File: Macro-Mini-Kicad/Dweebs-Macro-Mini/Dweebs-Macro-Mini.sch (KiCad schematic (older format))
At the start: 57 parts, among them U1 ProMicro

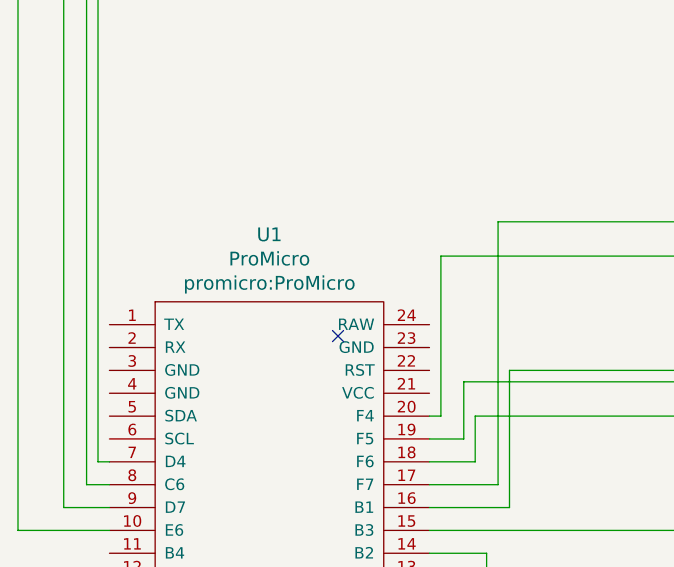
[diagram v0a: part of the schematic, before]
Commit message: more crap
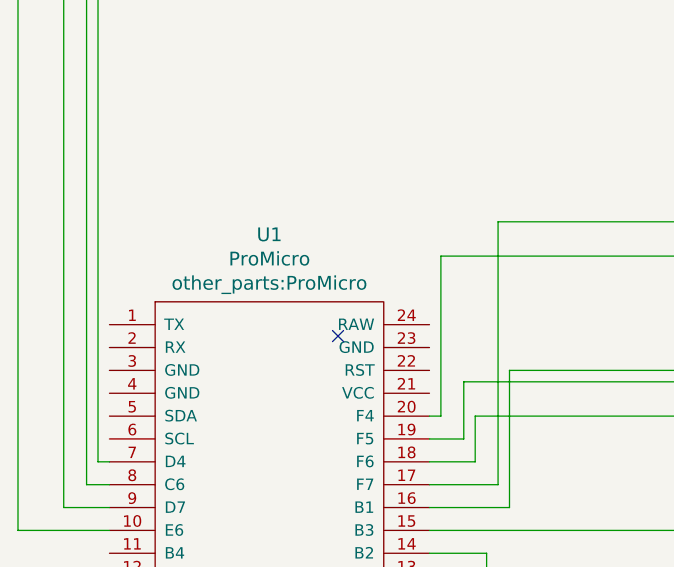
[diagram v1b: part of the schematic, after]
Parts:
- MX1, MX10, MX11, MX12, MX13, MX14, MX15, MX16, MX17, MX18, MX19, MX2, MX20, MX21, MX22, MX23, MX24, MX25, MX26, MX27, MX28, MX3, MX4, MX5, MX6, MX7, MX8, MX9: footprint MX_Alps_Hybrid:MX-1U-NoLED -> kbd:CherryMX_1u
- U1: footprint promicro:ProMicro -> other_parts:ProMicro
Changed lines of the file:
@@
 EESchema Schematic File Version 4
+LIBS:Dweebs-Macro-Mini-cache
 EELAYER 30 0
 EELAYER END
@@
 F 0 "MX1" H 4833 2073 60  0000 C CNN
 F 1 "MX-NoLED" H 4833 1999 20  0000 C CNN
-F 2 "MX_Alps_Hybrid:MX-1U-NoLED" H 4175 1825 60  0001 C CNN
+F 2 "kbd:CherryMX_1u" H 4175 1825 60  0001 C CNN
 F 3 "" H 4175 1825 60  0001 C CNN
 	1    4800 1850
@@
 F 0 "MX2" H 5233 2073 60  0000 C CNN
 F 1 "MX-NoLED" H 5233 1999 20  0000 C CNN
-F 2 "MX_Alps_Hybrid:MX-1U-NoLED" H 4575 1825 60  0001 C CNN
+F 2 "kbd:CherryMX_1u" H 4575 1825 60  0001 C CNN
 F 3 "" H 4575 1825 60  0001 C CNN
 	1    5200 1850
@@
 F 0 "MX3" H 5633 2073 60  0000 C CNN
 F 1 "MX-NoLED" H 5633 1999 20  0000 C CNN
-F 2 "MX_Alps_Hybrid:MX-1U-NoLED" H 4975 1825 60  0001 C CNN
+F 2 "kbd:CherryMX_1u" H 4975 1825 60  0001 C CNN
 F 3 "" H 4975 1825 60  0001 C CNN
 	1    5600 1850
@@
 F 0 "MX4" H 6033 2073 60  0000 C CNN
 F 1 "MX-NoLED" H 6033 1999 20  0000 C CNN
-F 2 "MX_Alps_Hybrid:MX-1U-NoLED" H 5375 1825 60  0001 C CNN
+F 2 "kbd:CherryMX_1u" H 5375 1825 60  0001 C CNN
 F 3 "" H 5375 1825 60  0001 C CNN
 	1    6000 1850
@@
 F 0 "MX5" H 6433 2073 60  0000 C CNN
 F 1 "MX-NoLED" H 6433 1999 20  0000 C CNN
-F 2 "MX_Alps_Hybrid:MX-1U-NoLED" H 5775 1825 60  0001 C CNN
+F 2 "kbd:CherryMX_1u" H 5775 1825 60  0001 C CNN
 F 3 "" H 5775 1825 60  0001 C CNN
 	1    6400 1850
@@
 F 0 "MX6" H 6833 2073 60  0000 C CNN
 F 1 "MX-NoLED" H 6833 1999 20  0000 C CNN
-F 2 "MX_Alps_Hybrid:MX-1U-NoLED" H 6175 1825 60  0001 C CNN
+F 2 "kbd:CherryMX_1u" H 6175 1825 60  0001 C CNN
 F 3 "" H 6175 1825 60  0001 C CNN
 	1    6800 1850
@@
 F 0 "MX7" H 7233 2073 60  0000 C CNN
 F 1 "MX-NoLED" H 7233 1999 20  0000 C CNN
-F 2 "MX_Alps_Hybrid:MX-1U-NoLED" H 6575 1825 60  0001 C CNN
+F 2 "kbd:CherryMX_1u" H 6575 1825 60  0001 C CNN
 F 3 "" H 6575 1825 60  0001 C CNN
 	1    7200 1850
@@
 F 0 "MX8" H 4833 2723 60  0000 C CNN
 F 1 "MX-NoLED" H 4833 2649 20  0000 C CNN
-F 2 "MX_Alps_Hybrid:MX-1U-NoLED" H 4175 2475 60  0001 C CNN
+F 2 "kbd:CherryMX_1u" H 4175 2475 60  0001 C CNN
 F 3 "" H 4175 2475 60  0001 C CNN
 	1    4800 2500
@@
 F 0 "MX9" H 5233 2723 60  0000 C CNN
 F 1 "MX-NoLED" H 5233 2649 20  0000 C CNN
-F 2 "MX_Alps_Hybrid:MX-1U-NoLED" H 4575 2475 60  0001 C CNN
+F 2 "kbd:CherryMX_1u" H 4575 2475 60  0001 C CNN
 F 3 "" H 4575 2475 60  0001 C CNN
 	1    5200 2500
@@
 F 0 "MX10" H 5633 2723 60  0000 C CNN
 F 1 "MX-NoLED" H 5633 2649 20  0000 C CNN
-F 2 "MX_Alps_Hybrid:MX-1U-NoLED" H 4975 2475 60  0001 C CNN
+F 2 "kbd:CherryMX_1u" H 4975 2475 60  0001 C CNN
 F 3 "" H 4975 2475 60  0001 C CNN
 	1    5600 2500
@@
 F 0 "MX11" H 6033 2723 60  0000 C CNN
 F 1 "MX-NoLED" H 6033 2649 20  0000 C CNN
-F 2 "MX_Alps_Hybrid:MX-1U-NoLED" H 5375 2475 60  0001 C CNN
+F 2 "kbd:CherryMX_1u" H 5375 2475 60  0001 C CNN
 F 3 "" H 5375 2475 60  0001 C CNN
 	1    6000 2500
@@
 F 0 "MX12" H 6433 2723 60  0000 C CNN
 F 1 "MX-NoLED" H 6433 2649 20  0000 C CNN
-F 2 "MX_Alps_Hybrid:MX-1U-NoLED" H 5775 2475 60  0001 C CNN
+F 2 "kbd:CherryMX_1u" H 5775 2475 60  0001 C CNN
 F 3 "" H 5775 2475 60  0001 C CNN
 	1    6400 2500
@@
 F 0 "MX13" H 6833 2723 60  0000 C CNN
 F 1 "MX-NoLED" H 6833 2649 20  0000 C CNN
-F 2 "MX_Alps_Hybrid:MX-1U-NoLED" H 6175 2475 60  0001 C CNN
+F 2 "kbd:CherryMX_1u" H 6175 2475 60  0001 C CNN
 F 3 "" H 6175 2475 60  0001 C CNN
 	1    6800 2500
@@
 F 0 "MX14" H 4833 3423 60  0000 C CNN
 F 1 "MX-NoLED" H 4833 3349 20  0000 C CNN
-F 2 "MX_Alps_Hybrid:MX-1U-NoLED" H 4175 3175 60  0001 C CNN
+F 2 "kbd:CherryMX_1u" H 4175 3175 60  0001 C CNN
 F 3 "" H 4175 3175 60  0001 C CNN
 	1    4800 3200
@@
 F 0 "MX15" H 5233 3423 60  0000 C CNN
 F 1 "MX-NoLED" H 5233 3349 20  0000 C CNN
-F 2 "MX_Alps_Hybrid:MX-1U-NoLED" H 4575 3175 60  0001 C CNN
+F 2 "kbd:CherryMX_1u" H 4575 3175 60  0001 C CNN
 F 3 "" H 4575 3175 60  0001 C CNN
 	1    5200 3200
@@
 F 0 "MX16" H 5633 3423 60  0000 C CNN
 F 1 "MX-NoLED" H 5633 3349 20  0000 C CNN
-F 2 "MX_Alps_Hybrid:MX-1U-NoLED" H 4975 3175 60  0001 C CNN
+F 2 "kbd:CherryMX_1u" H 4975 3175 60  0001 C CNN
 F 3 "" H 4975 3175 60  0001 C CNN
 	1    5600 3200
@@
 F 0 "MX17" H 6033 3423 60  0000 C CNN
 F 1 "MX-NoLED" H 6033 3349 20  0000 C CNN
-F 2 "MX_Alps_Hybrid:MX-1U-NoLED" H 5375 3175 60  0001 C CNN
+F 2 "kbd:CherryMX_1u" H 5375 3175 60  0001 C CNN
 F 3 "" H 5375 3175 60  0001 C CNN
 	1    6000 3200
@@
 F 0 "MX18" H 6433 3423 60  0000 C CNN
 F 1 "MX-NoLED" H 6433 3349 20  0000 C CNN
-F 2 "MX_Alps_Hybrid:MX-1U-NoLED" H 5775 3175 60  0001 C CNN
+F 2 "kbd:CherryMX_1u" H 5775 3175 60  0001 C CNN
 F 3 "" H 5775 3175 60  0001 C CNN
 	1    6400 3200
@@
 F 0 "MX19" H 6833 3423 60  0000 C CNN
 F 1 "MX-NoLED" H 6833 3349 20  0000 C CNN
-F 2 "MX_Alps_Hybrid:MX-1U-NoLED" H 6175 3175 60  0001 C CNN
+F 2 "kbd:CherryMX_1u" H 6175 3175 60  0001 C CNN
 F 3 "" H 6175 3175 60  0001 C CNN
 	1    6800 3200
@@
 F 0 "MX20" H 4833 4073 60  0000 C CNN
 F 1 "MX-NoLED" H 4833 3999 20  0000 C CNN
-F 2 "MX_Alps_Hybrid:MX-1U-NoLED" H 4175 3825 60  0001 C CNN
+F 2 "kbd:CherryMX_1u" H 4175 3825 60  0001 C CNN
 F 3 "" H 4175 3825 60  0001 C CNN
 	1    4800 3850
@@
 F 0 "MX21" H 5233 4073 60  0000 C CNN
 F 1 "MX-NoLED" H 5233 3999 20  0000 C CNN
-F 2 "MX_Alps_Hybrid:MX-1U-NoLED" H 4575 3825 60  0001 C CNN
+F 2 "kbd:CherryMX_1u" H 4575 3825 60  0001 C CNN
 F 3 "" H 4575 3825 60  0001 C CNN
 	1    5200 3850
@@
 F 0 "MX22" H 5633 4073 60  0000 C CNN
 F 1 "MX-NoLED" H 5633 3999 20  0000 C CNN
-F 2 "MX_Alps_Hybrid:MX-1U-NoLED" H 4975 3825 60  0001 C CNN
+F 2 "kbd:CherryMX_1u" H 4975 3825 60  0001 C CNN
 F 3 "" H 4975 3825 60  0001 C CNN
 	1    5600 3850
@@
 F 0 "MX23" H 6033 4073 60  0000 C CNN
 F 1 "MX-NoLED" H 6033 3999 20  0000 C CNN
-F 2 "MX_Alps_Hybrid:MX-1U-NoLED" H 5375 3825 60  0001 C CNN
+F 2 "kbd:CherryMX_1u" H 5375 3825 60  0001 C CNN
 F 3 "" H 5375 3825 60  0001 C CNN
 	1    6000 3850
@@
 F 0 "MX24" H 6433 4073 60  0000 C CNN
 F 1 "MX-NoLED" H 6433 3999 20  0000 C CNN
-F 2 "MX_Alps_Hybrid:MX-1U-NoLED" H 5775 3825 60  0001 C CNN
+F 2 "kbd:CherryMX_1u" H 5775 3825 60  0001 C CNN
 F 3 "" H 5775 3825 60  0001 C CNN
 	1    6400 3850
@@
 F 0 "MX25" H 6833 4073 60  0000 C CNN
 F 1 "MX-NoLED" H 6833 3999 20  0000 C CNN
-F 2 "MX_Alps_Hybrid:MX-1U-NoLED" H 6175 3825 60  0001 C CNN
+F 2 "kbd:CherryMX_1u" H 6175 3825 60  0001 C CNN
 F 3 "" H 6175 3825 60  0001 C CNN
 	1    6800 3850
@@
 F 0 "MX26" H 4833 4723 60  0000 C CNN
 F 1 "MX-NoLED" H 4833 4649 20  0000 C CNN
-F 2 "MX_Alps_Hybrid:MX-1U-NoLED" H 4175 4475 60  0001 C CNN
+F 2 "kbd:CherryMX_1u" H 4175 4475 60  0001 C CNN
 F 3 "" H 4175 4475 60  0001 C CNN
 	1    4800 4500
@@
 F 0 "MX27" H 5233 4723 60  0000 C CNN
 F 1 "MX-NoLED" H 5233 4649 20  0000 C CNN
-F 2 "MX_Alps_Hybrid:MX-1U-NoLED" H 4575 4475 60  0001 C CNN
+F 2 "kbd:CherryMX_1u" H 4575 4475 60  0001 C CNN
 F 3 "" H 4575 4475 60  0001 C CNN
 	1    5200 4500
@@
 F 0 "MX28" H 5633 4723 60  0000 C CNN
 F 1 "MX-NoLED" H 5633 4649 20  0000 C CNN
-F 2 "MX_Alps_Hybrid:MX-1U-NoLED" H 4975 4475 60  0001 C CNN
+F 2 "kbd:CherryMX_1u" H 4975 4475 60  0001 C CNN
 F 3 "" H 4975 4475 60  0001 C CNN
 	1    5600 4500
@@
 F 0 "U1" H 2000 4543 60  0000 C CNN
 F 1 "ProMicro" H 2000 4437 60  0000 C CNN
-F 2 "promicro:ProMicro" H 2000 4331 60  0000 C CNN
+F 2 "other_parts:ProMicro" H 2000 4331 60  0000 C CNN
 F 3 "" H 2100 2350 60  0000 C CNN
 	1    2000 3400

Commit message: change
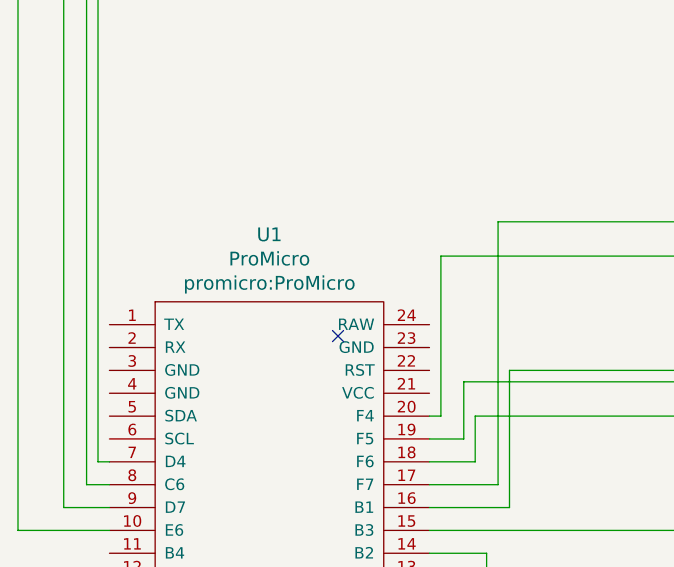
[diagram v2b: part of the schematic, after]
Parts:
- MX1, MX10, MX11, MX12, MX13, MX14, MX15, MX16, MX17, MX18, MX19, MX2, MX20, MX21, MX22, MX23, MX24, MX25, MX26, MX27, MX28, MX3, MX4, MX5, MX6, MX7, MX8, MX9: footprint kbd:CherryMX_1u -> MX_Alps_Hybrid:MX-1U-NoLED
- U1: footprint other_parts:ProMicro -> promicro:ProMicro
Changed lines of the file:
@@
 F 0 "MX1" H 4833 2073 60  0000 C CNN
 F 1 "MX-NoLED" H 4833 1999 20  0000 C CNN
-F 2 "kbd:CherryMX_1u" H 4175 1825 60  0001 C CNN
+F 2 "MX_Alps_Hybrid:MX-1U-NoLED" H 4175 1825 60  0001 C CNN
 F 3 "" H 4175 1825 60  0001 C CNN
 	1    4800 1850
@@
 F 0 "MX2" H 5233 2073 60  0000 C CNN
 F 1 "MX-NoLED" H 5233 1999 20  0000 C CNN
-F 2 "kbd:CherryMX_1u" H 4575 1825 60  0001 C CNN
+F 2 "MX_Alps_Hybrid:MX-1U-NoLED" H 4575 1825 60  0001 C CNN
 F 3 "" H 4575 1825 60  0001 C CNN
 	1    5200 1850
@@
 F 0 "MX3" H 5633 2073 60  0000 C CNN
 F 1 "MX-NoLED" H 5633 1999 20  0000 C CNN
-F 2 "kbd:CherryMX_1u" H 4975 1825 60  0001 C CNN
+F 2 "MX_Alps_Hybrid:MX-1U-NoLED" H 4975 1825 60  0001 C CNN
 F 3 "" H 4975 1825 60  0001 C CNN
 	1    5600 1850
@@
 F 0 "MX4" H 6033 2073 60  0000 C CNN
 F 1 "MX-NoLED" H 6033 1999 20  0000 C CNN
-F 2 "kbd:CherryMX_1u" H 5375 1825 60  0001 C CNN
+F 2 "MX_Alps_Hybrid:MX-1U-NoLED" H 5375 1825 60  0001 C CNN
 F 3 "" H 5375 1825 60  0001 C CNN
 	1    6000 1850
@@
 F 0 "MX5" H 6433 2073 60  0000 C CNN
 F 1 "MX-NoLED" H 6433 1999 20  0000 C CNN
-F 2 "kbd:CherryMX_1u" H 5775 1825 60  0001 C CNN
+F 2 "MX_Alps_Hybrid:MX-1U-NoLED" H 5775 1825 60  0001 C CNN
 F 3 "" H 5775 1825 60  0001 C CNN
 	1    6400 1850
@@
 F 0 "MX6" H 6833 2073 60  0000 C CNN
 F 1 "MX-NoLED" H 6833 1999 20  0000 C CNN
-F 2 "kbd:CherryMX_1u" H 6175 1825 60  0001 C CNN
+F 2 "MX_Alps_Hybrid:MX-1U-NoLED" H 6175 1825 60  0001 C CNN
 F 3 "" H 6175 1825 60  0001 C CNN
 	1    6800 1850
@@
 F 0 "MX7" H 7233 2073 60  0000 C CNN
 F 1 "MX-NoLED" H 7233 1999 20  0000 C CNN
-F 2 "kbd:CherryMX_1u" H 6575 1825 60  0001 C CNN
+F 2 "MX_Alps_Hybrid:MX-1U-NoLED" H 6575 1825 60  0001 C CNN
 F 3 "" H 6575 1825 60  0001 C CNN
 	1    7200 1850
@@
 F 0 "MX8" H 4833 2723 60  0000 C CNN
 F 1 "MX-NoLED" H 4833 2649 20  0000 C CNN
-F 2 "kbd:CherryMX_1u" H 4175 2475 60  0001 C CNN
+F 2 "MX_Alps_Hybrid:MX-1U-NoLED" H 4175 2475 60  0001 C CNN
 F 3 "" H 4175 2475 60  0001 C CNN
 	1    4800 2500
@@
 F 0 "MX9" H 5233 2723 60  0000 C CNN
 F 1 "MX-NoLED" H 5233 2649 20  0000 C CNN
-F 2 "kbd:CherryMX_1u" H 4575 2475 60  0001 C CNN
+F 2 "MX_Alps_Hybrid:MX-1U-NoLED" H 4575 2475 60  0001 C CNN
 F 3 "" H 4575 2475 60  0001 C CNN
 	1    5200 2500
@@
 F 0 "MX10" H 5633 2723 60  0000 C CNN
 F 1 "MX-NoLED" H 5633 2649 20  0000 C CNN
-F 2 "kbd:CherryMX_1u" H 4975 2475 60  0001 C CNN
+F 2 "MX_Alps_Hybrid:MX-1U-NoLED" H 4975 2475 60  0001 C CNN
 F 3 "" H 4975 2475 60  0001 C CNN
 	1    5600 2500
@@
 F 0 "MX11" H 6033 2723 60  0000 C CNN
 F 1 "MX-NoLED" H 6033 2649 20  0000 C CNN
-F 2 "kbd:CherryMX_1u" H 5375 2475 60  0001 C CNN
+F 2 "MX_Alps_Hybrid:MX-1U-NoLED" H 5375 2475 60  0001 C CNN
 F 3 "" H 5375 2475 60  0001 C CNN
 	1    6000 2500
@@
 F 0 "MX12" H 6433 2723 60  0000 C CNN
 F 1 "MX-NoLED" H 6433 2649 20  0000 C CNN
-F 2 "kbd:CherryMX_1u" H 5775 2475 60  0001 C CNN
+F 2 "MX_Alps_Hybrid:MX-1U-NoLED" H 5775 2475 60  0001 C CNN
 F 3 "" H 5775 2475 60  0001 C CNN
 	1    6400 2500
@@
 F 0 "MX13" H 6833 2723 60  0000 C CNN
 F 1 "MX-NoLED" H 6833 2649 20  0000 C CNN
-F 2 "kbd:CherryMX_1u" H 6175 2475 60  0001 C CNN
+F 2 "MX_Alps_Hybrid:MX-1U-NoLED" H 6175 2475 60  0001 C CNN
 F 3 "" H 6175 2475 60  0001 C CNN
 	1    6800 2500
@@
 F 0 "MX14" H 4833 3423 60  0000 C CNN
 F 1 "MX-NoLED" H 4833 3349 20  0000 C CNN
-F 2 "kbd:CherryMX_1u" H 4175 3175 60  0001 C CNN
+F 2 "MX_Alps_Hybrid:MX-1U-NoLED" H 4175 3175 60  0001 C CNN
 F 3 "" H 4175 3175 60  0001 C CNN
 	1    4800 3200
@@
 F 0 "MX15" H 5233 3423 60  0000 C CNN
 F 1 "MX-NoLED" H 5233 3349 20  0000 C CNN
-F 2 "kbd:CherryMX_1u" H 4575 3175 60  0001 C CNN
+F 2 "MX_Alps_Hybrid:MX-1U-NoLED" H 4575 3175 60  0001 C CNN
 F 3 "" H 4575 3175 60  0001 C CNN
 	1    5200 3200
@@
 F 0 "MX16" H 5633 3423 60  0000 C CNN
 F 1 "MX-NoLED" H 5633 3349 20  0000 C CNN
-F 2 "kbd:CherryMX_1u" H 4975 3175 60  0001 C CNN
+F 2 "MX_Alps_Hybrid:MX-1U-NoLED" H 4975 3175 60  0001 C CNN
 F 3 "" H 4975 3175 60  0001 C CNN
 	1    5600 3200
@@
 F 0 "MX17" H 6033 3423 60  0000 C CNN
 F 1 "MX-NoLED" H 6033 3349 20  0000 C CNN
-F 2 "kbd:CherryMX_1u" H 5375 3175 60  0001 C CNN
+F 2 "MX_Alps_Hybrid:MX-1U-NoLED" H 5375 3175 60  0001 C CNN
 F 3 "" H 5375 3175 60  0001 C CNN
 	1    6000 3200
@@
 F 0 "MX18" H 6433 3423 60  0000 C CNN
 F 1 "MX-NoLED" H 6433 3349 20  0000 C CNN
-F 2 "kbd:CherryMX_1u" H 5775 3175 60  0001 C CNN
+F 2 "MX_Alps_Hybrid:MX-1U-NoLED" H 5775 3175 60  0001 C CNN
 F 3 "" H 5775 3175 60  0001 C CNN
 	1    6400 3200
@@
 F 0 "MX19" H 6833 3423 60  0000 C CNN
 F 1 "MX-NoLED" H 6833 3349 20  0000 C CNN
-F 2 "kbd:CherryMX_1u" H 6175 3175 60  0001 C CNN
+F 2 "MX_Alps_Hybrid:MX-1U-NoLED" H 6175 3175 60  0001 C CNN
 F 3 "" H 6175 3175 60  0001 C CNN
 	1    6800 3200
@@
 F 0 "MX20" H 4833 4073 60  0000 C CNN
 F 1 "MX-NoLED" H 4833 3999 20  0000 C CNN
-F 2 "kbd:CherryMX_1u" H 4175 3825 60  0001 C CNN
+F 2 "MX_Alps_Hybrid:MX-1U-NoLED" H 4175 3825 60  0001 C CNN
 F 3 "" H 4175 3825 60  0001 C CNN
 	1    4800 3850
@@
 F 0 "MX21" H 5233 4073 60  0000 C CNN
 F 1 "MX-NoLED" H 5233 3999 20  0000 C CNN
-F 2 "kbd:CherryMX_1u" H 4575 3825 60  0001 C CNN
+F 2 "MX_Alps_Hybrid:MX-1U-NoLED" H 4575 3825 60  0001 C CNN
 F 3 "" H 4575 3825 60  0001 C CNN
 	1    5200 3850
@@
 F 0 "MX22" H 5633 4073 60  0000 C CNN
 F 1 "MX-NoLED" H 5633 3999 20  0000 C CNN
-F 2 "kbd:CherryMX_1u" H 4975 3825 60  0001 C CNN
+F 2 "MX_Alps_Hybrid:MX-1U-NoLED" H 4975 3825 60  0001 C CNN
 F 3 "" H 4975 3825 60  0001 C CNN
 	1    5600 3850
@@
 F 0 "MX23" H 6033 4073 60  0000 C CNN
 F 1 "MX-NoLED" H 6033 3999 20  0000 C CNN
-F 2 "kbd:CherryMX_1u" H 5375 3825 60  0001 C CNN
+F 2 "MX_Alps_Hybrid:MX-1U-NoLED" H 5375 3825 60  0001 C CNN
 F 3 "" H 5375 3825 60  0001 C CNN
 	1    6000 3850
@@
 F 0 "MX24" H 6433 4073 60  0000 C CNN
 F 1 "MX-NoLED" H 6433 3999 20  0000 C CNN
-F 2 "kbd:CherryMX_1u" H 5775 3825 60  0001 C CNN
+F 2 "MX_Alps_Hybrid:MX-1U-NoLED" H 5775 3825 60  0001 C CNN
 F 3 "" H 5775 3825 60  0001 C CNN
 	1    6400 3850
@@
 F 0 "MX25" H 6833 4073 60  0000 C CNN
 F 1 "MX-NoLED" H 6833 3999 20  0000 C CNN
-F 2 "kbd:CherryMX_1u" H 6175 3825 60  0001 C CNN
+F 2 "MX_Alps_Hybrid:MX-1U-NoLED" H 6175 3825 60  0001 C CNN
 F 3 "" H 6175 3825 60  0001 C CNN
 	1    6800 3850
@@
 F 0 "MX26" H 4833 4723 60  0000 C CNN
 F 1 "MX-NoLED" H 4833 4649 20  0000 C CNN
-F 2 "kbd:CherryMX_1u" H 4175 4475 60  0001 C CNN
+F 2 "MX_Alps_Hybrid:MX-1U-NoLED" H 4175 4475 60  0001 C CNN
 F 3 "" H 4175 4475 60  0001 C CNN
 	1    4800 4500
@@
 F 0 "MX27" H 5233 4723 60  0000 C CNN
 F 1 "MX-NoLED" H 5233 4649 20  0000 C CNN
-F 2 "kbd:CherryMX_1u" H 4575 4475 60  0001 C CNN
+F 2 "MX_Alps_Hybrid:MX-1U-NoLED" H 4575 4475 60  0001 C CNN
 F 3 "" H 4575 4475 60  0001 C CNN
 	1    5200 4500
@@
 F 0 "MX28" H 5633 4723 60  0000 C CNN
 F 1 "MX-NoLED" H 5633 4649 20  0000 C CNN
-F 2 "kbd:CherryMX_1u" H 4975 4475 60  0001 C CNN
+F 2 "MX_Alps_Hybrid:MX-1U-NoLED" H 4975 4475 60  0001 C CNN
 F 3 "" H 4975 4475 60  0001 C CNN
 	1    5600 4500
@@
 F 0 "U1" H 2000 4543 60  0000 C CNN
 F 1 "ProMicro" H 2000 4437 60  0000 C CNN
-F 2 "other_parts:ProMicro" H 2000 4331 60  0000 C CNN
+F 2 "promicro:ProMicro" H 2000 4331 60  0000 C CNN
 F 3 "" H 2100 2350 60  0000 C CNN
 	1    2000 3400
